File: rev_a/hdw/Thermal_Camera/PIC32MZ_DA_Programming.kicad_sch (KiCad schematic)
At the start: 17 parts

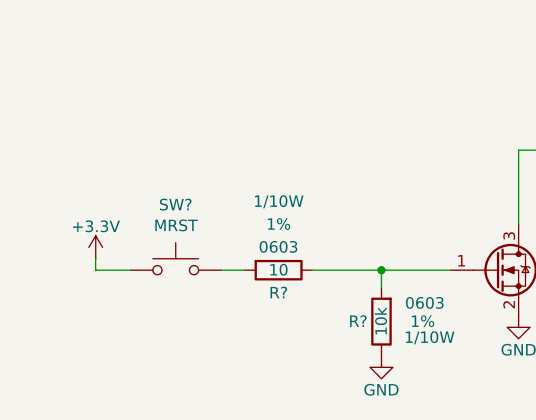
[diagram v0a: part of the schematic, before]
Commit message: added some power supplies
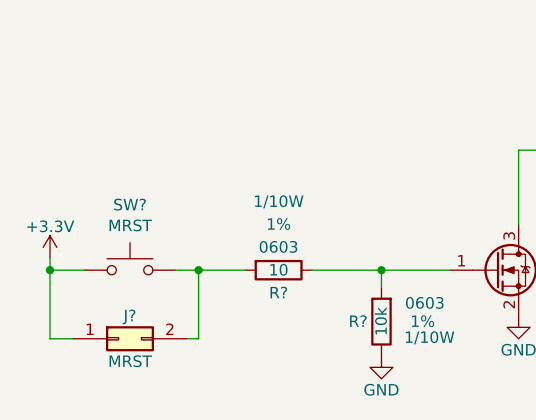
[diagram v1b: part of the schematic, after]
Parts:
- added J?: MRST, symbol Connector_Generic:Conn_02x01
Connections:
- net +3.3V: now also J?.1 (Pin_1)
- net at R?.1, SW?.2: now also J?.2 (Pin_2)
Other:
- moved on the sheet: SW?
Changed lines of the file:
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@@
     (company "Drew Maatman and Michael Laffin")
   )
+  (junction (at 69.85 139.7) (diameter 0) (color 0 0 0 0)
+  )
   (junction (at 106.68 139.7) (diameter 0) (color 0 0 0 0)
+  )
+  (junction (at 86.36 139.7) (diameter 0) (color 0 0 0 0)
   )
   (junction (at 96.52 49.53) (diameter 0) (color 0 0 0 0)
@@
     (stroke (width 0) (type default))
   )
+  (wire (pts (xy 86.36 139.7) (xy 83.82 139.7))
+    (stroke (width 0) (type default))
+  )
   (wire (pts (xy 102.87 71.12) (xy 102.87 54.61))
     (stroke (width 0) (type default))
@@
     (stroke (width 0) (type default))
   )
+  (wire (pts (xy 86.36 139.7) (xy 86.36 147.32))
+    (stroke (width 0) (type default))
+  )
   (wire (pts (xy 90.17 71.12) (xy 90.17 46.99))
     (stroke (width 0) (type default))
@@
     (stroke (width 0) (type default))
   )
+  (wire (pts (xy 72.39 147.32) (xy 69.85 147.32))
+    (stroke (width 0) (type default))
+  )
   (wire (pts (xy 135.255 52.07) (xy 176.53 52.07))
     (stroke (width 0) (type default))
@@
     (stroke (width 0) (type default))
   )
-  (wire (pts (xy 74.93 139.7) (xy 78.74 139.7))
+  (wire (pts (xy 85.09 147.32) (xy 86.36 147.32))
+    (stroke (width 0) (type default))
+  )
+  (wire (pts (xy 69.85 139.7) (xy 73.66 139.7))
     (stroke (width 0) (type default))
   )
@@
     (stroke (width 0) (type default))
   )
+  (wire (pts (xy 69.85 147.32) (xy 69.85 139.7))
+    (stroke (width 0) (type default))
+  )
   (wire (pts (xy 134.62 126.365) (xy 147.955 126.365))
     (stroke (width 0) (type default))
   )
-  (wire (pts (xy 74.93 138.43) (xy 74.93 139.7))
-    (stroke (width 0) (type default))
-  )
-  (wire (pts (xy 91.44 139.7) (xy 88.9 139.7))
+  (wire (pts (xy 69.85 138.43) (xy 69.85 139.7))
+    (stroke (width 0) (type default))
+  )
+  (wire (pts (xy 91.44 139.7) (xy 86.36 139.7))
     (stroke (width 0) (type default))
   )
@@
     )
   )
-  (symbol (lib_id "Switch:SW_Push") (at 83.82 139.7 0) (unit 1)
-    (in_bom yes) (on_board yes) (dnp no)
-    (property "Reference" "SW?" (at 83.82 132.461 0)
-      (effects (font (size 1.27 1.27)))
-    )
-    (property "Value" "MRST" (at 83.82 134.7724 0)
-      (effects (font (size 1.27 1.27)))
-    )
-    (property "Footprint" "Button_Switch_THT:SW_PUSH_6mm" (at 83.82 134.62 0)
-      (effects (font (size 1.27 1.27)) hide)
-    )
-    (property "Datasheet" "" (at 83.82 134.62 0)
+  (symbol (lib_id "Switch:SW_Push") (at 78.74 139.7 0) (unit 1)
+    (in_bom yes) (on_board yes) (dnp no)
+    (property "Reference" "SW?" (at 78.74 132.461 0)
+      (effects (font (size 1.27 1.27)))
+    )
+    (property "Value" "MRST" (at 78.74 134.7724 0)
+      (effects (font (size 1.27 1.27)))
+    )
+    (property "Footprint" "Button_Switch_THT:SW_PUSH_6mm" (at 78.74 134.62 0)
+      (effects (font (size 1.27 1.27)) hide)
+    )
+    (property "Datasheet" "" (at 78.74 134.62 0)
       (effects (font (size 1.27 1.27)) hide)
     )
@@
         (path "/4bd21e0b-5408-4b93-866e-c82ac5b31fa9/c8b41008-ee29-40ae-a4f4-13001b750237"
           (reference "SW?") (unit 1)
+        )
+      )
+    )
+  )
+  (symbol (lib_id "Connector_Generic:Conn_02x01") (at 77.47 147.32 0) (unit 1)
+    (in_bom yes) (on_board yes) (dnp no)
+    (property "Reference" "J?" (at 78.74 144.78 0)
+      (effects (font (size 1.27 1.27)))
+    )
+    (property "Value" "MRST" (at 78.74 149.86 0)
+      (effects (font (size 1.27 1.27)))
+    )
+    (property "Footprint" "" (at 77.47 147.32 0)
+      (effects (font (size 1.27 1.27)) hide)
+    )
+    (property "Datasheet" "~" (at 77.47 147.32 0)
+      (effects (font (size 1.27 1.27)) hide)
+    )
+    (pin "2")
+    (pin "1")
+    (instances
+      (project "Thermal_Camera"
+        (path "/4bd21e0b-5408-4b93-866e-c82ac5b31fa9/c8b41008-ee29-40ae-a4f4-13001b750237"
+          (reference "J?") (unit 1)
         )
       )
@@
     )
   )
-  (symbol (lib_id "power:+3.3V") (at 74.93 138.43 0) (unit 1)
-    (in_bom yes) (on_board yes) (dnp no)
-    (property "Reference" "#PWR?" (at 74.93 142.24 0)
-      (effects (font (size 1.27 1.27)) hide)
-    )
-    (property "Value" "+3.3V" (at 74.93 134.874 0)
-      (effects (font (size 1.27 1.27)))
-    )
-    (property "Footprint" "" (at 74.93 138.43 0)
-      (effects (font (size 1.27 1.27)) hide)
-    )
-    (property "Datasheet" "" (at 74.93 138.43 0)
-      (effects (font (size 1.27 1.27)) hide)
-    )
+  (symbol (lib_id "power:+3.3V") (at 69.85 138.43 0) (unit 1)
+    (in_bom yes) (on_board yes) (dnp no)
+    (property "Reference" "#PWR?" (at 69.85 142.24 0)
+      (effects (font (size 1.27 1.27)) hide)
+    )
+    (property "Value" "+3.3V" (at 69.85 134.874 0)
+      (effects (font (size 1.27 1.27)))
+    )
+    (property "Footprint" "" (at 69.85 138.43 0)
+      (effects (font (size 1.27 1.27)) hide)
+    )
+    (property "Datasheet" "" (at 69.85 138.43 0)
+      (effects (font (size 1.27 1.27)) hide)
+    )
